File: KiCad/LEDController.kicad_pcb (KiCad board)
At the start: 4 copper layers, 50 x 50 mm, 40 parts, among them J1 Conn_01x05, J2 UART, J3 JTAG, J5 USB_C_Receptacle_USB2.0_16P, J6 Conn_01x03, J7 VDD, J8 GND, J9 Conn_01x14, Q1 IRLZ44N, Q2 IRLZ44N, Q3 IRLZ44N, Q4 IRLZ44N, SW1 BOOT, SW2 ENABLE, U1 TPS62132, U2 ESP32-S3-WROOM-2

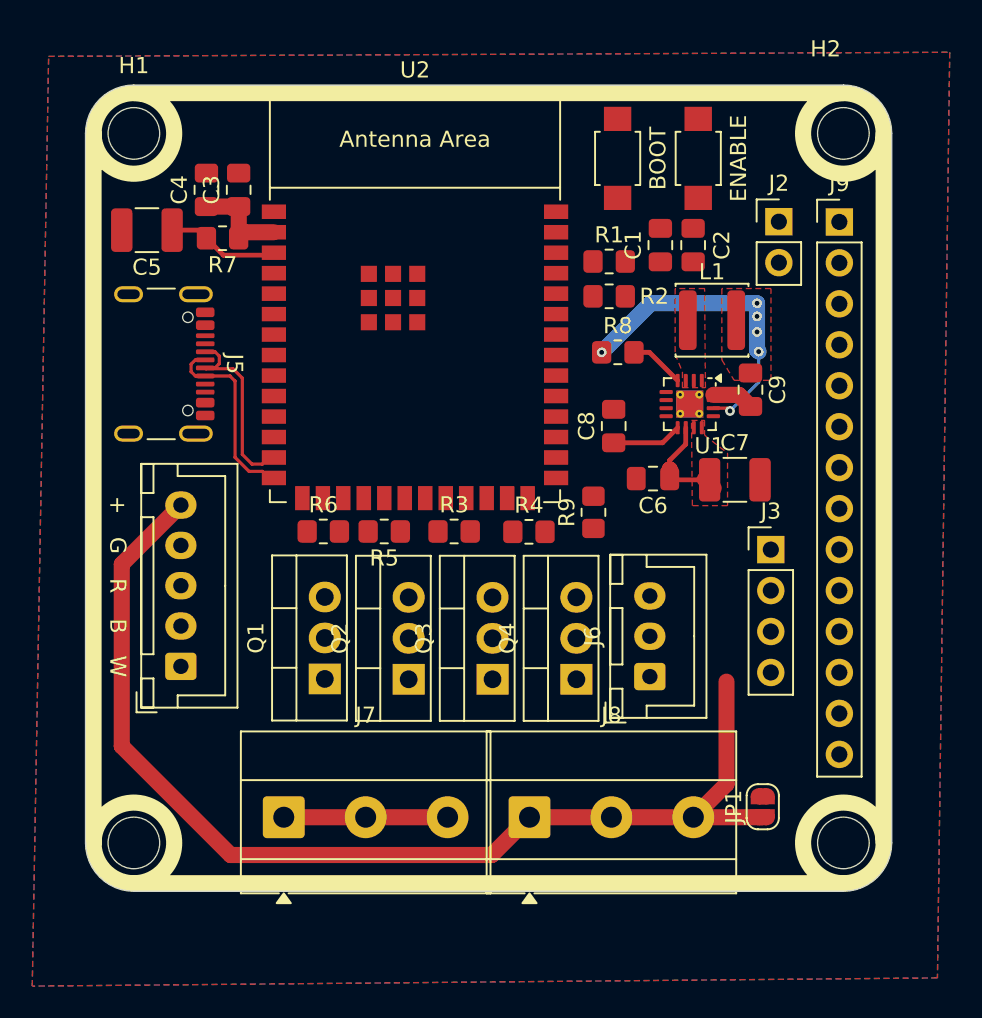
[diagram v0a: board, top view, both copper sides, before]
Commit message: .
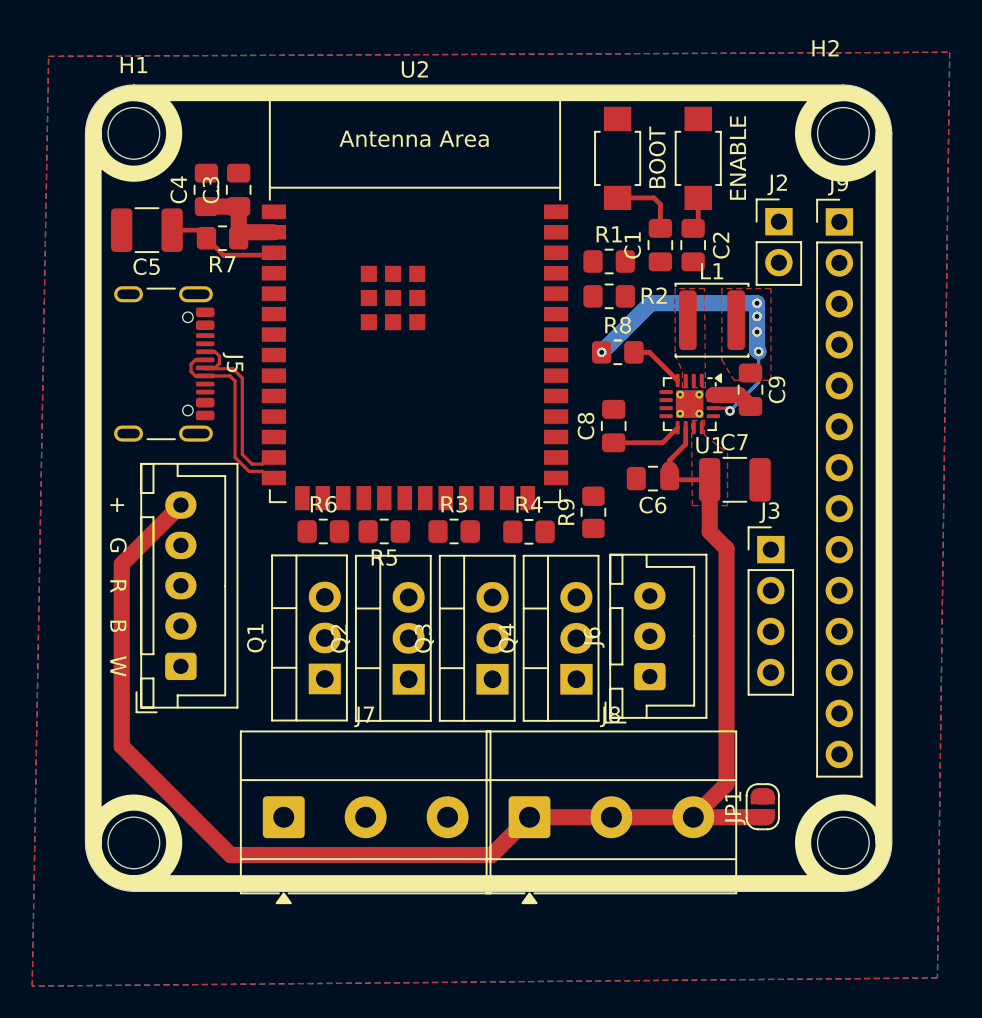
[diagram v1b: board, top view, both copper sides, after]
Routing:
- net +24V: track 76.7 -> 88.9 mm
- net GND: track 12.8 -> 2.60 mm
- net ESP_BOOT: track 0.00 -> 4.31 mm
- net ESP_EN: track 7.02 -> 9.04 mm
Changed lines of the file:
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@@
+	)
+	(segment
+		(start 124.75 77.75)
+		(end 123.7085 76.7085)
+		(width 1)
+		(locked yes)
+		(layer "F.Cu")
+		(net 1)
 	)
 	(segment
@@
 	)
 	(segment
+		(start 123.7085 76.7085)
+		(end 123.7085 73.483)
+		(width 1)
+		(locked yes)
+		(layer "F.Cu")
+		(net 1)
+	)
+	(segment
 		(start 112.535 94.4065)
 		(end 110.1915 96.75)
@@
 	)
 	(segment
+		(start 121.2303 73.4063)
+		(end 121.2303 73.406)
+		(width 1)
+		(locked yes)
+		(layer "F.Cu")
+		(net 1)
+	)
+	(segment
 		(start 110.1915 96.75)
 		(end 94 96.75)
@@
 	)
 	(segment
-		(start 124.75 92.3515)
-		(end 124.75 86)
-		(width 1)
-		(locked yes)
-		(layer "F.Cu")
-		(net 1)
-	)
-	(segment
 		(start 121.2303 73.406)
 		(end 121.2303 72.2669)
@@
 	)
 	(segment
+		(start 124.75 92.3515)
+		(end 124.75 77.75)
+		(width 1)
+		(locked yes)
+		(layer "F.Cu")
+		(net 1)
+	)
+	(segment
 		(start 121.2303 72.8367)
 		(end 121.2303 73.406)
@@
 	)
 	(segment
-		(start 123.4043 73.4482)
-		(end 123.9556 73.9995)
-		(width 1)
-		(locked yes)
-		(layer "F.Cu")
-		(net 1)
-	)
-	(segment
-		(start 97.295 94.4065)
-		(end 107.455 94.4065)
-		(width 1)
-		(layer "F.Cu")
-		(net 2)
+		(start 121.2685 73.4445)
+		(end 121.2303 73.4063)
+		(width 1)
+		(locked yes)
+		(layer "F.Cu")
+		(net 1)
 	)
 	(segment
@@
 	)
 	(segment
+		(start 123 56)
+		(end 123 57.5725)
+		(width 0.3)
+		(locked yes)
+		(layer "F.Cu")
+		(net 5)
+	)
+	(segment
 		(start 96.531 59.551)
 		(end 96.684 59.398)
@@
 		(layer "F.Cu")
 		(net 5)
+	)
+	(segment
+		(start 123 57.5725)
+		(end 122.682 57.8905)
+		(width 0.3)
+		(locked yes)
+		(layer "F.Cu")
+		(net 5)
+	)
+	(segment
+		(start 120.65 56.4)
+		(end 120.65 57.8905)
+		(width 0.3)
+		(locked yes)
+		(layer "F.Cu")
+		(net 6)
+	)
+	(segment
+		(start 118 56)
+		(end 120.25 56)
+		(width 0.3)
+		(locked yes)
+		(layer "F.Cu")
+		(net 6)
+	)
+	(segment
+		(start 120.25 56)
+		(end 120.65 56.4)
+		(width 0.3)
+		(locked yes)
+		(layer "F.Cu")
+		(net 6)
 	)
 	(segment
@@
 		)
 	)
-	(group ""
-		(locked yes)
-		(members "01828b56-34e0-4a06-a3bf-28ad11a34c5a" "1c7e8a6f-f2f5-4e6d-a802-88a13df24168"
-			"21bdb9d8-bf2f-453b-bcd4-2856f7a4a413" "457147a2-ef18-45b0-b280-cf6765241b55"
-			"46141387-b783-4eca-88e7-9b1fef433324" "5a9325b2-5d57-4d75-b5a9-3242ae65519b"
-			"692bf279-3e98-42e2-8c72-cc135f14818b" "84f42245-9690-4e30-ae27-08fc111fd4a3"
-			"92405c58-db03-4148-bb69-0bfeaf815f0a" "94ee00f1-81c6-40c2-9a85-2dcfd6776d02"
-			"a7e7a91f-8641-4af0-b3ef-a454fbc7569a" "a94018c4-9228-4e0f-9750-be65928fefcd"
-			"aa58f986-5f5b-482f-8677-e671ee6c0a88" "ae2c4346-d1d5-498d-81ad-7d7f909279ac"
-			"b9324584-4b93-42a0-baa1-b42d30034026" "c2ba79c6-28e2-4018-99fe-8b7b30e6304f"
-			"c2ca5805-b247-466d-9a6d-d8db4c54b930" "c3204412-d963-4cae-af26-e04c5b9c5683"
-			"c5f66cfd-3a2a-411a-af6f-0376a95c4a74" "d210df41-780c-4e85-82f6-d132ecebb21c"
-			"d22ce7e1-464b-41e7-a746-925fdb4bc739" "d59aea36-8e0b-4e55-a1ef-fd7072b163ae"
-			"dc29fb80-82c3-42fd-8468-10d0b983914a" "dffcf38c-12da-4939-994c-b450ebcf85a3"
-			"e88183c6-135c-484d-aca6-c18ac4f7a445" "ecdc397c-6dbc-4ad7-9db0-883d03c6996f"
-			"efce23ec-90b2-498e-bf46-94fa4c1abbe8" "f69433e8-45e1-4a71-8aa0-e3f665ab8def"
-			"f856bc97-eb50-4a21-896d-e43ce4389c5f" "ffae4f2f-3083-49c5-b2c9-3705d5b3ecf3"
-		)
-	)
